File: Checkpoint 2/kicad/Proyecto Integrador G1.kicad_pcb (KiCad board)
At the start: 2 copper layers, 82.6 x 76.9 mm, 50 parts, among them J1 Conn_01x02, J2 Conn_01x02, Q1 BC547, Q10 BC547, Q2 BC547, Q3 BC547, Q4 BC547, Q5 BC557, Q6 BC557, Q7 BC547, Q8 TIP42C, Q9 BC547, U1 TL431LP, U2 LM358

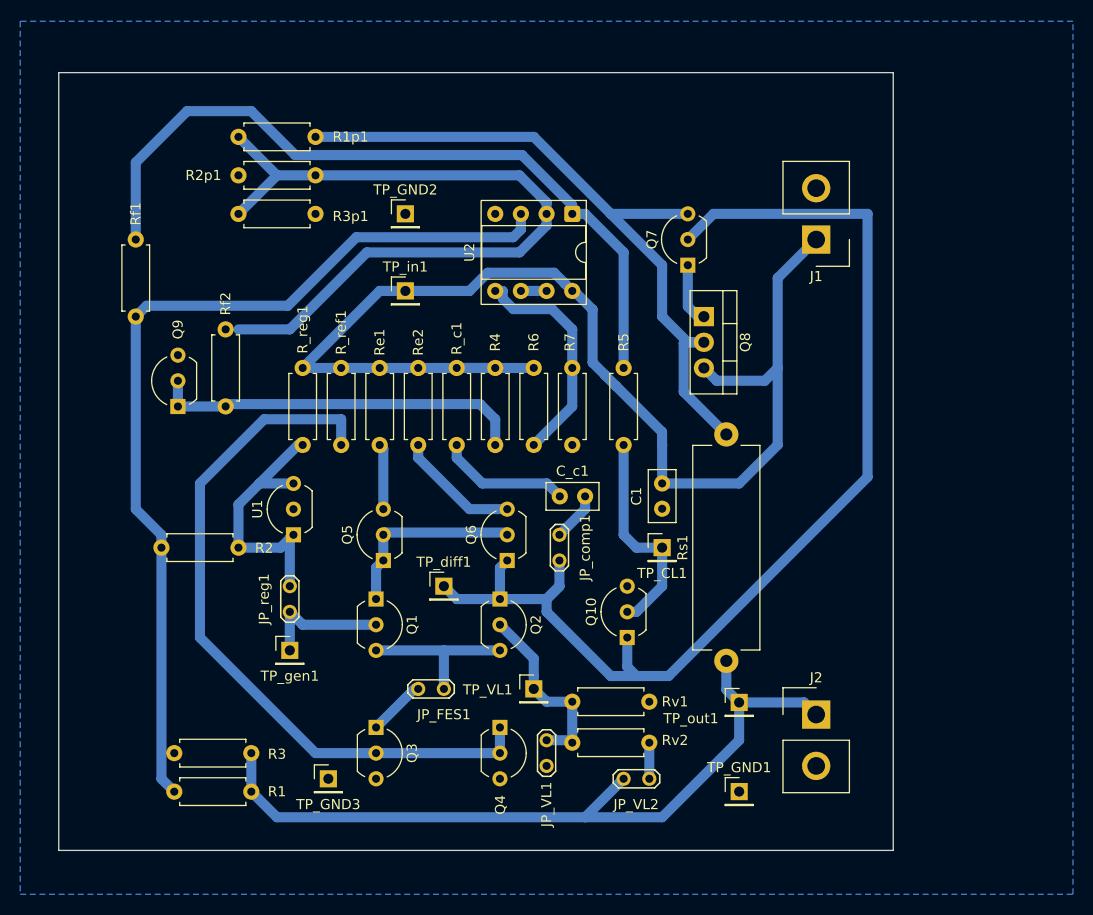
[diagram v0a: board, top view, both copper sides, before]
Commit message: rev 1.1
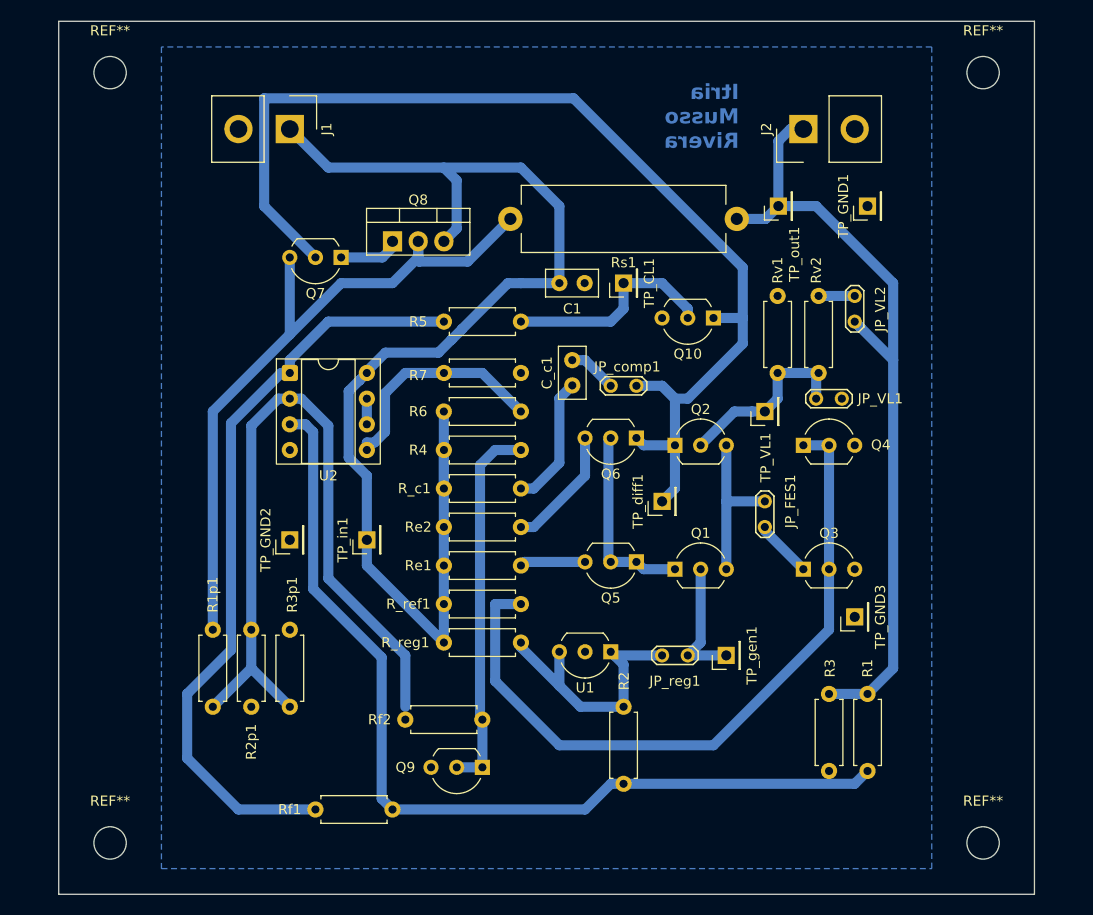
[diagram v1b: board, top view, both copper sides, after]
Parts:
- added REF**: MountingHole_3.2mm_M3, MountingHole:MountingHole_3.2mm_M3, F.Cu at (116.8, 99.1)
- added REF**: MountingHole_3.2mm_M3, MountingHole:MountingHole_3.2mm_M3, F.Cu at (116.8, 22.9)
- added REF**: MountingHole_3.2mm_M3, MountingHole:MountingHole_3.2mm_M3, F.Cu at (30.5, 22.9)
- added REF**: MountingHole_3.2mm_M3, MountingHole:MountingHole_3.2mm_M3, F.Cu at (30.5, 99.1)
- moved R1 61.7 mm to (105.4, 84.3), turned to -90 degrees
- moved TP_GND1 59.3 mm to (105.4, 36.1), turned to 90 degrees
- moved Rf1 59.1 mm to (50.8, 95.8), turned to 0 degrees
- moved J2 57.9 mm to (99.1, 28.4), turned to 90 degrees
- moved R3 57.4 mm to (101.6, 84.3), turned to -90 degrees
- moved TP_GND3 54.5 mm to (104.1, 76.7), turned to 90 degrees
- moved J1 53.2 mm to (48.3, 28.4), turned to -90 degrees
- moved R2p1 52.6 mm to (44.4, 85.6), turned to 90 degrees
- moved JP_VL2 51.9 mm to (104.1, 45.0), turned to -90 degrees
- moved R1p1 49.8 mm to (40.6, 78.0), turned to -90 degrees
- moved TP_out1 49.3 mm to (96.6, 36.1), turned to 90 degrees
- moved Q9 46.7 mm to (67.3, 91.6), turned to 180 degrees
- moved JP_VL1 46.6 mm to (102.9, 55.1), turned to 180 degrees
- moved Q3 45.1 mm to (99.1, 72.0), turned to 0 degrees
- moved Rv2 43.9 mm to (100.6, 52.6), turned to 90 degrees
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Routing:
- net Vref: track 124.1 -> 126.6 mm
- net Vb: track 113.8 -> 112.5 mm
- net Vout: track 79.0 -> 80.3 mm
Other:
- board size 82.6 x 76.9 mm -> 96.5 x 86.4 mm
- board text added: "Itria Musso Rivera"
